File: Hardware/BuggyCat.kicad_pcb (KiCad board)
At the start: 2 copper layers, 36.8 x 104 mm, 104 parts, among them J1 Antenna, J2 BG306-02-A-2-0400-L-G, J3 Header7, J4 Header 2, J5 Header 4, J6 Input Power:2x AA Battery, P1 USB_C_Plug_USB2.0, Q1 AO3422, Q2 AO3422, Q3 LDA111STR, Q4 RGT16BM65DTL, Q5 DMG3415U-7, SW1 TL3342F450QG, SW2 ON, SW3 TL3342F450QG, SW4 RESET, SW5 BOOT, SW6 TL3342F450QG, T1 ATB322524, T2 ATB322524, U1 AP2112K-3.3, U2 W25Q16JV, U3 RP2040, Y1 12Mhz

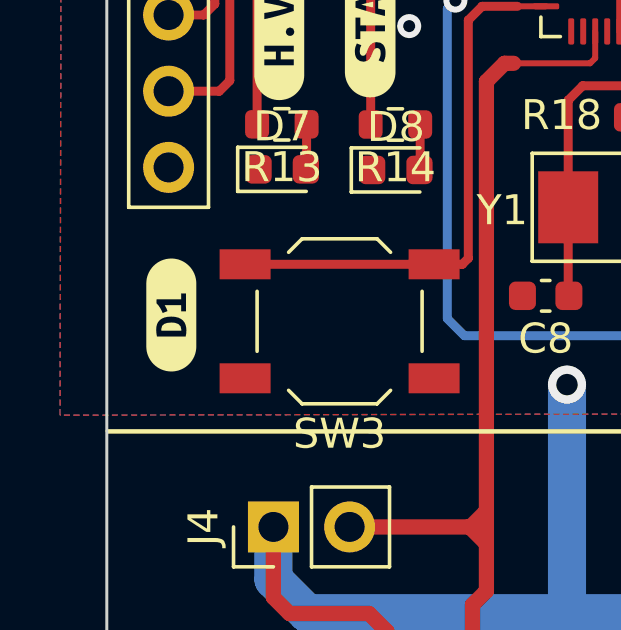
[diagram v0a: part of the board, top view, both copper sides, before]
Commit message: change label pulse
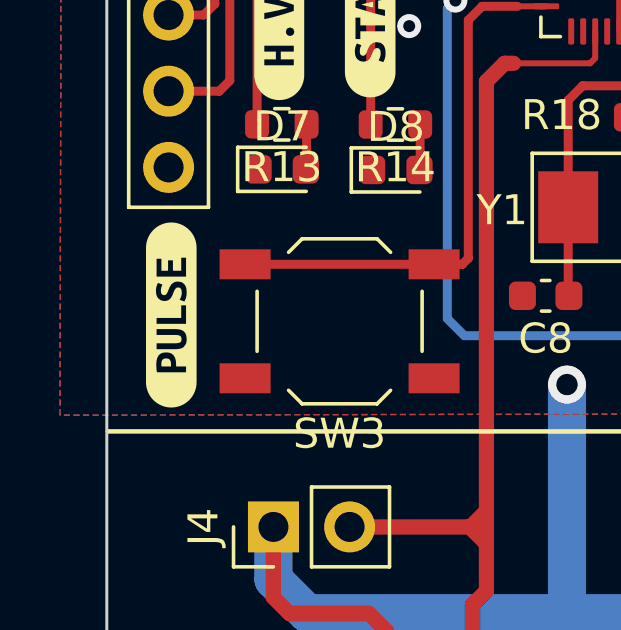
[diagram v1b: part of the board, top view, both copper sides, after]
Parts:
- removed kibuzzard-642DF795: G***, kibuzzard-642DF795
- added kibuzzard-642F0B74: G***, kibuzzard-642F0B74, F.Cu at (50.0, 58.9)
